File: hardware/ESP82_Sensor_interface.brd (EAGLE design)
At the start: 26.4 x 63.4 mm, 13 parts

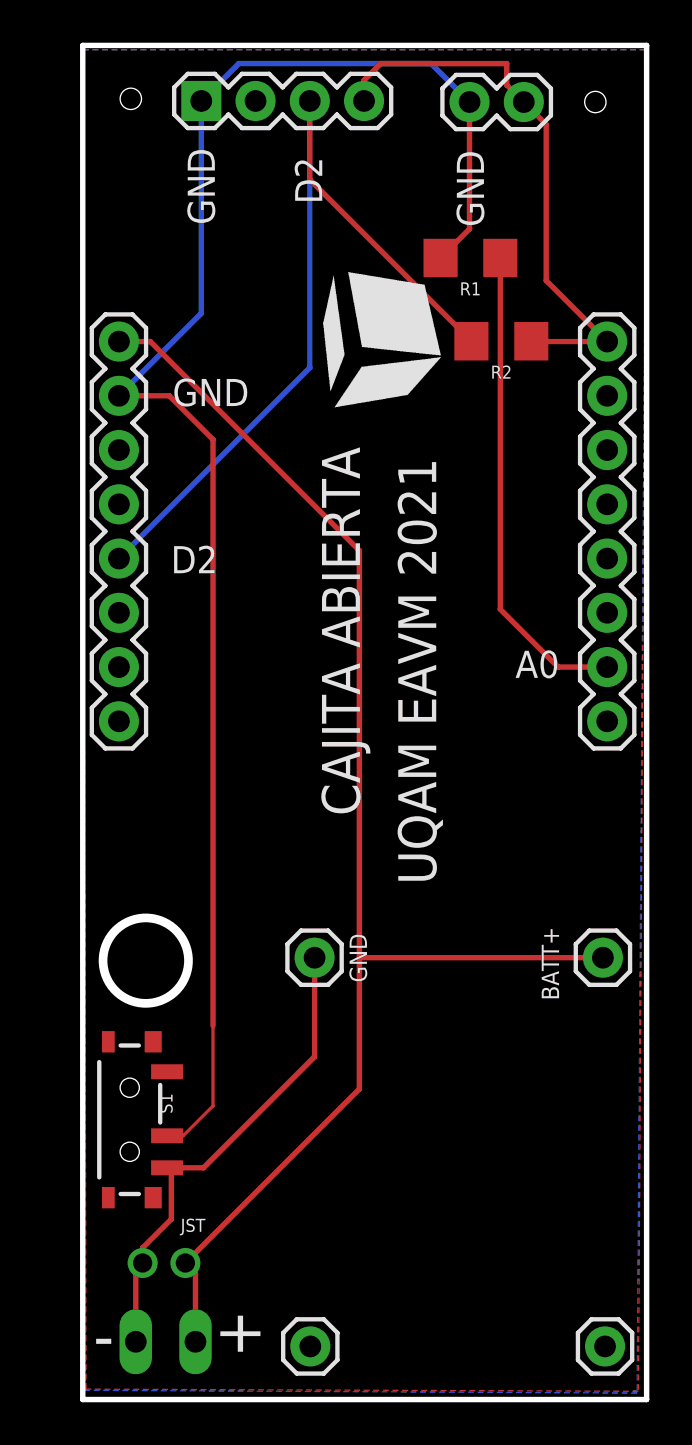
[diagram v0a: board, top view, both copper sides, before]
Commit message: new hardware version
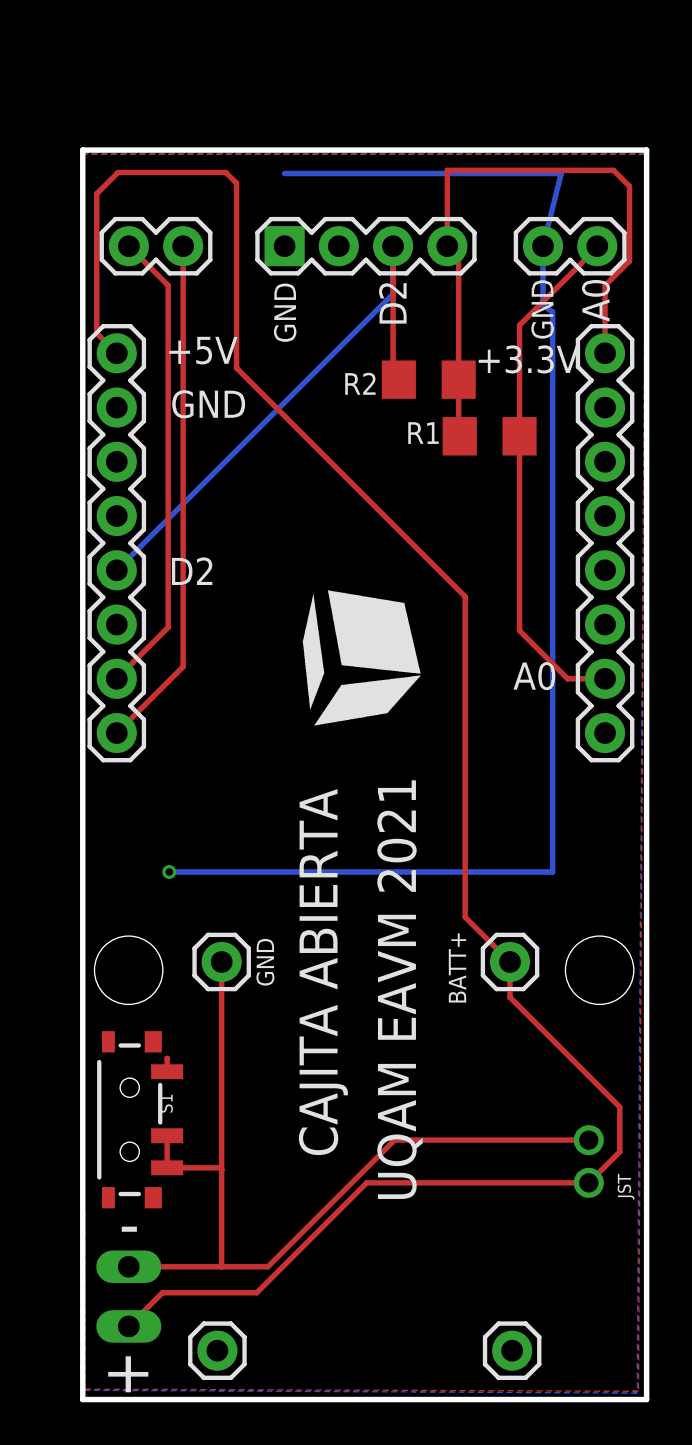
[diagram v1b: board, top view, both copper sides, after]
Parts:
- added SERIAL: (no value), SparkFun-Connectors:1X02
- added U$1, U$2: (no value), WingTechCorner:M3-HOLE
- WEMOS2: value Wemos D1 mini -> Wemos D1
- moved JST 20.4 mm to (23.7, 11.1), turned to 180 degrees
- moved R1 8.40 mm to (19.1, 45.1), turned to 0 degrees
- moved JP2 7.84 mm to (9.45, 54.0)
- moved JP1 6.81 mm to (21.6, 54.0), turned to 0 degrees
- moved BATT+ 4.35 mm to (20.0, 20.5)
- moved PIN0 4.35 mm to (20.1, 2.29)
- moved GND 4.35 mm to (6.50, 20.5)
- moved KK 4.35 mm to (6.30, 2.29)
- moved R2 3.85 mm to (16.2, 47.8)
- moved BATT 3.42 mm to (2.16, 6.09), turned to 270 degrees
- moved WEMOS1 0.56 mm to (24.5, 31.2)
- moved WEMOS2 0.56 mm to (1.59, 49.0)
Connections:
- new net RX: SERIAL.2, WEMOS2.7
- new net TX: SERIAL.1, WEMOS2.8
- net 3.3V: now also R1.1; no longer JP1.1
- net A0: now also JP1.2, R1.2; no longer R1.1
- net ENTREEGND: now also S1.2
- net GND: now also JP1.1, S1.3; no longer JP1.2, R1.2, S1.2
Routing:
- net 5V: track 67.3 -> 94.2 mm
- net TX: track 0.00 -> 24.1 mm
- net RX: track 0.00 -> 22.0 mm
- net ENTREEGND: track 22.6 -> 42.4 mm
- net D2: track 39.5 -> 27.1 mm
- net GND: track 76.5 -> 64.7 mm, vias 0 -> 1
- net 3.3V: track 26.5 -> 30.1 mm
- net A0: track 22.6 -> 24.4 mm
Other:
- board size 26.4 x 63.4 mm -> 26.4 x 58.5 mm
- board text added: "3.3V"
- board text added: "RX"
- board text added: "TX"
- board text removed: "D1"
- board text removed: "D5"
- board text removed: "D6"
